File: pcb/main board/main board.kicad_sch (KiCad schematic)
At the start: 46 parts, among them J10 12V Battery, J11 BAU, J12 Servo 4 Conn, J13 Servo 1 Conn, J14 Servo 2 Conn, J15 Servo 3 Conn, J16 Servo 5 Conn, J17 Servo 6 Conn, J18 Servo 7 Conn, J19 Servo 8 Conn, J20 Motor 1 Encoder, J21 Motor 2 Encoder, J22 Motor 3 Encoder, J23 Motor 4 Encoder, J24 Fan 1 Conn, J25 Fan 2 Conn, J5 I2C 0 Conn, J6 I2C 1 Conn, Q1 IRF8714PBF, Q2 IRF8714PBF, U4 MCP23017_SO, U6 LM3150MH

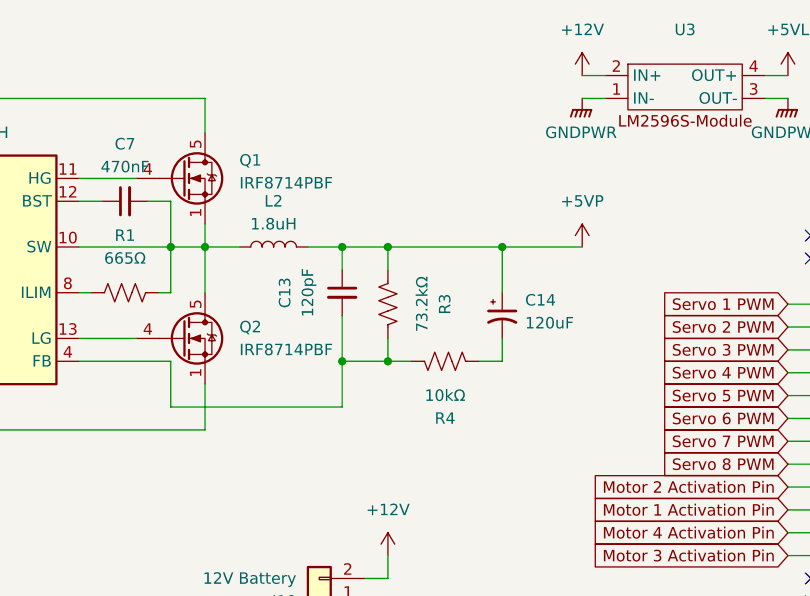
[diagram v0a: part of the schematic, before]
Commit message: Updated PCB and corrected errors
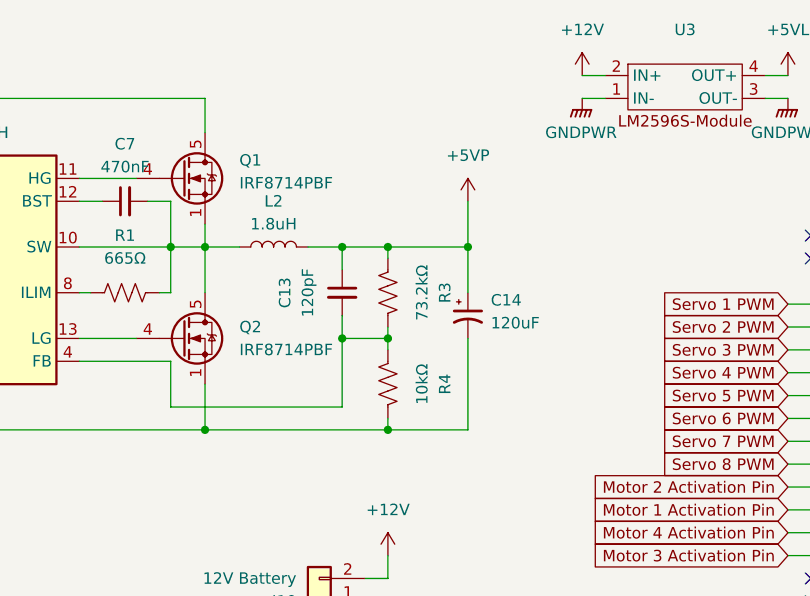
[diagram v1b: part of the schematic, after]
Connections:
- net GNDPWR: now also C14.2, R4.1
- net at C13.2, R3.1, U6.4 (FB): now also R4.2; no longer R4.1
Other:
- moved on the sheet: C14, R3, R4
